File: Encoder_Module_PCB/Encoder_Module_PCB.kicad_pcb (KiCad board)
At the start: 2 copper layers, 4 parts, among them J3 Enc_Enc_01x06, U9 AS5048A-HTSP

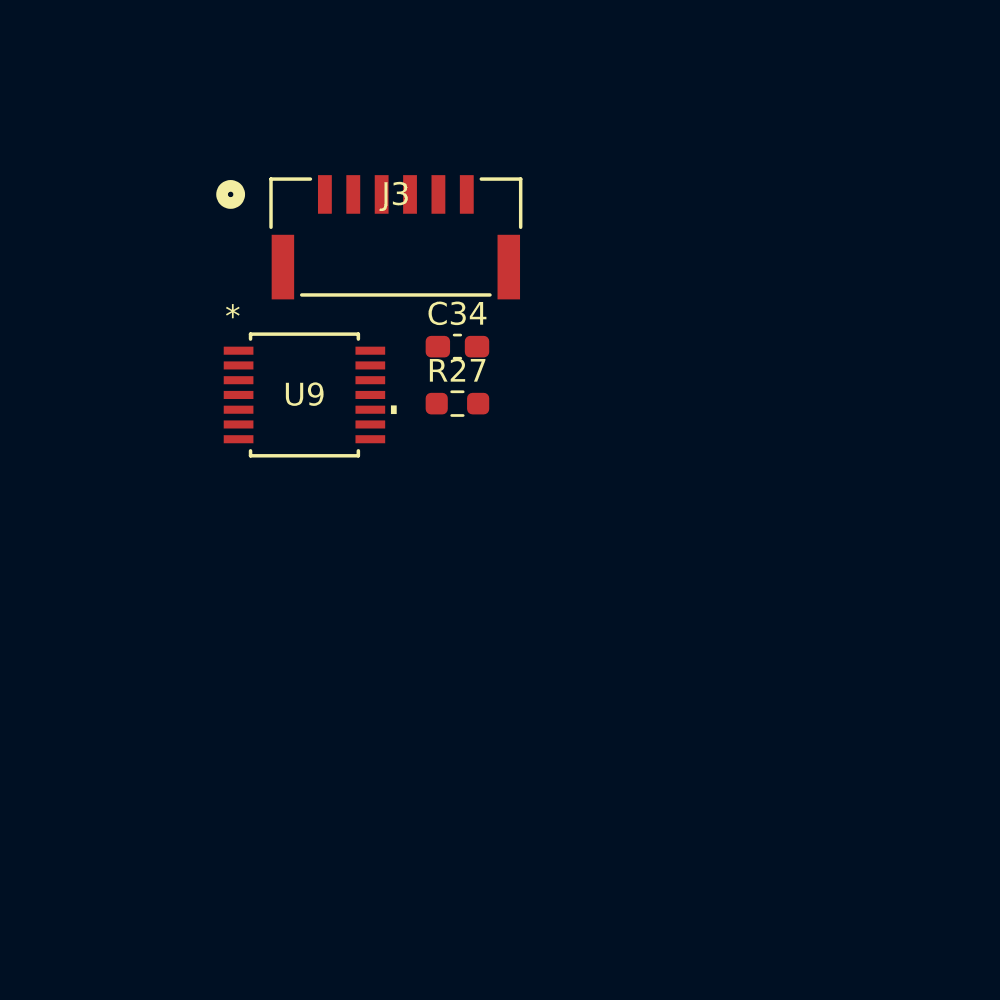
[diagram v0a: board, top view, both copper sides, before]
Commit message: rearranged some file and directories
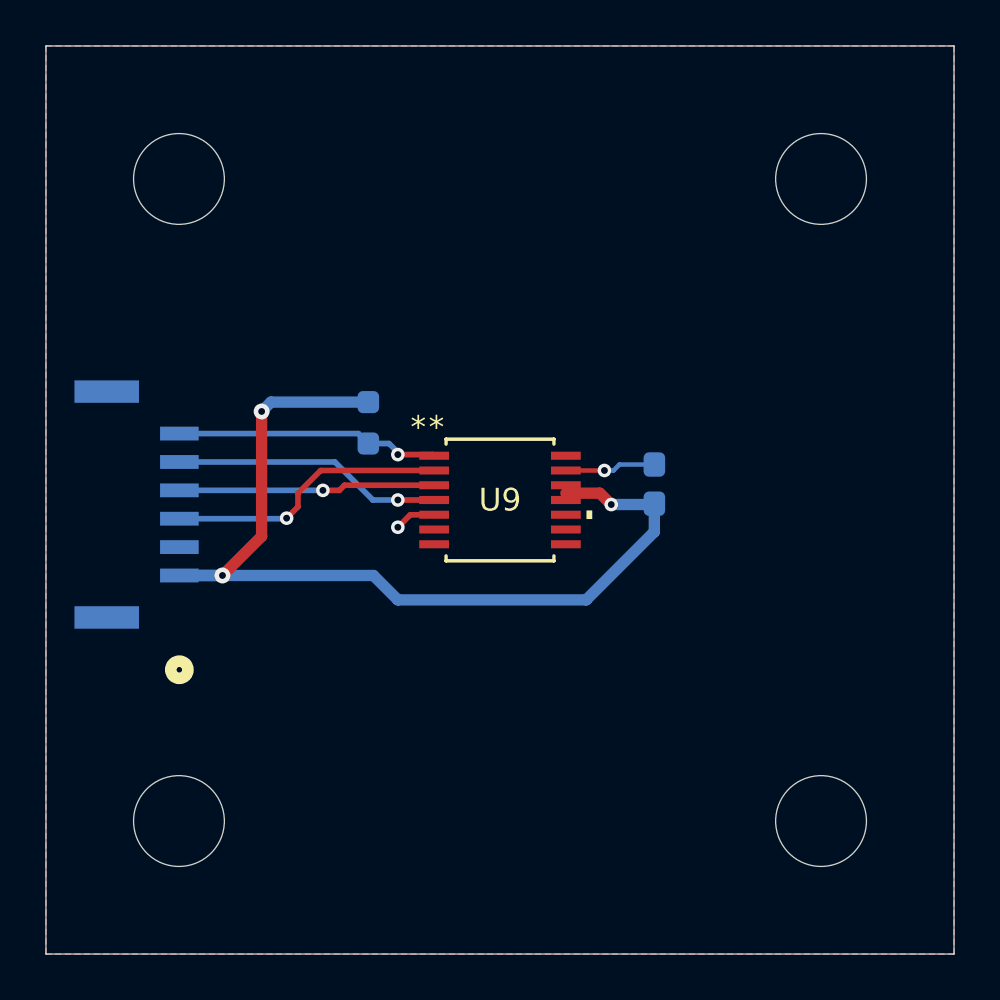
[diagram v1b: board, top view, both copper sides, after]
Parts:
- added REF**: MountingHole_4mm, MountingHole:MountingHole_4mm, F.Cu at (164.1, 75.9)
- added REF**: MountingHole_4mm, MountingHole:MountingHole_4mm, F.Cu at (164.1, 104.1)
- added REF**: MountingHole_4mm, MountingHole:MountingHole_4mm, F.Cu at (135.9, 75.9)
- added REF**: MountingHole_4mm, MountingHole:MountingHole_4mm, F.Cu at (135.9, 104.1)
- C34, J3, R27: moved to B.Cu
- moved J3 16.4 mm to (134.0, 90.2), turned to 90 degrees
- moved C34 10.6 mm to (156.8, 89.3), turned to 90 degrees
- moved U9 9.78 mm to (150.0, 90.0)
- moved R27 4.01 mm to (144.2, 86.6), turned to -90 degrees
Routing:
- net ENC_+3.3V: track 0.00 -> 43.3 mm, vias 0 -> 3
- net SCLK_ENC: track 0.00 -> 12.5 mm, vias 0 -> 1
- net SDI_ENC: track 0.00 -> 11.9 mm, vias 0 -> 1
- net SCS_ENC: track 0.00 -> 11.7 mm, vias 0 -> 1
- net SDO_ENC: track 0.00 -> 11.3 mm, vias 0 -> 1
- net GND_ENC: track 0.00 -> 5.83 mm, vias 0 -> 2
- added copper zone on B.Cu, net GND_ENC
- added copper zone on F.Cu, net GND_ENC
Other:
- board outline added: 40 x 40 mm
